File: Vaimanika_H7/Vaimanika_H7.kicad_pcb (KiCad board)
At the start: 4 copper layers, 40 x 40 mm, 64 parts, among them CN1 WAFER-GH1.25-3PWB, J1 TYPE-C 16PIN 2MD, J2 Conn_01x09, J3 Conn_01x09, J4 +VLIPO, J5 GND, J6 Conn_01x09, J8 Conn_01x02, Q1 AO3400A, Q2 AO3401A, U2 TPS54302, U3 USBLC6-2P6, U4 WAFER-GH1.25-4PWB, U5 WAFER-GH1.25-4PWB, U6 WAFER-GH1.25-4PWB, U7 WAFER-GH1.25-4PLB, U8 WAFER-GH1.25-4PLB, U9 WAFER-GH1.25-4PLB

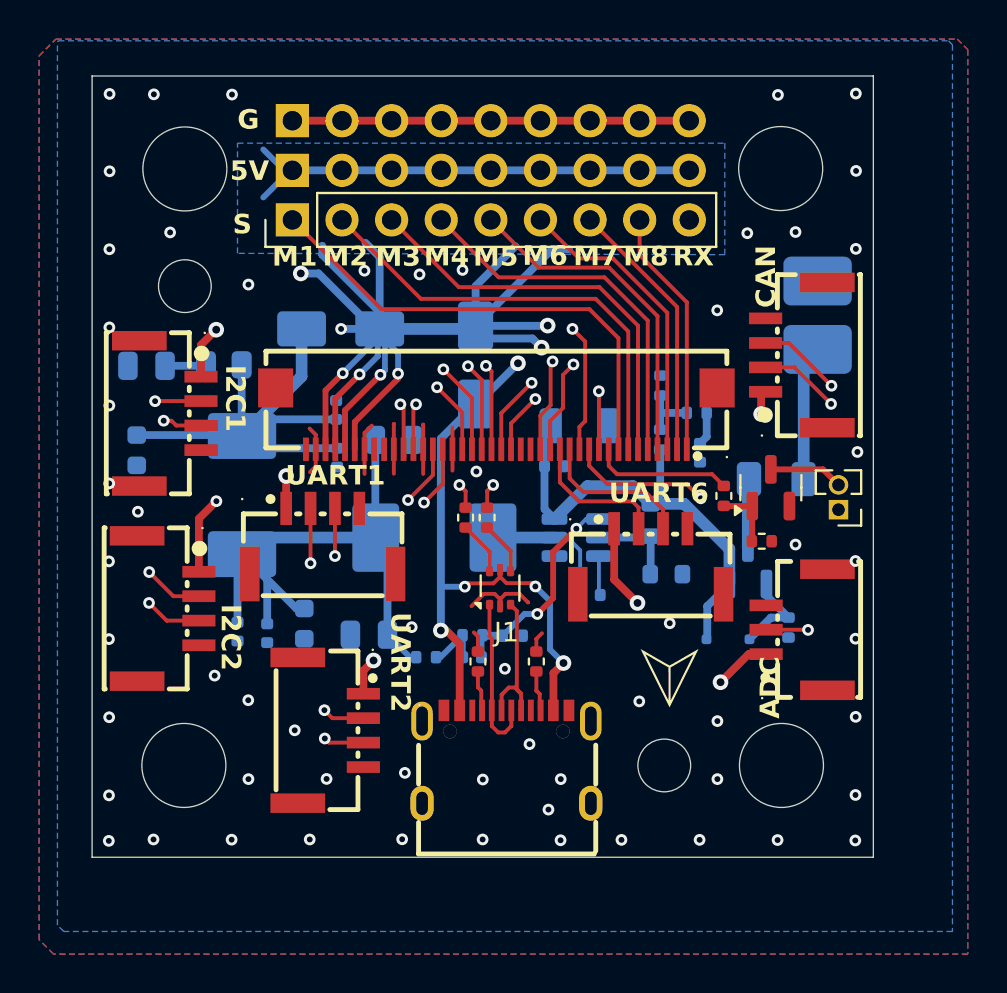
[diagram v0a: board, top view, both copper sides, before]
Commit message: Pilot PCB Done/03-06-2026
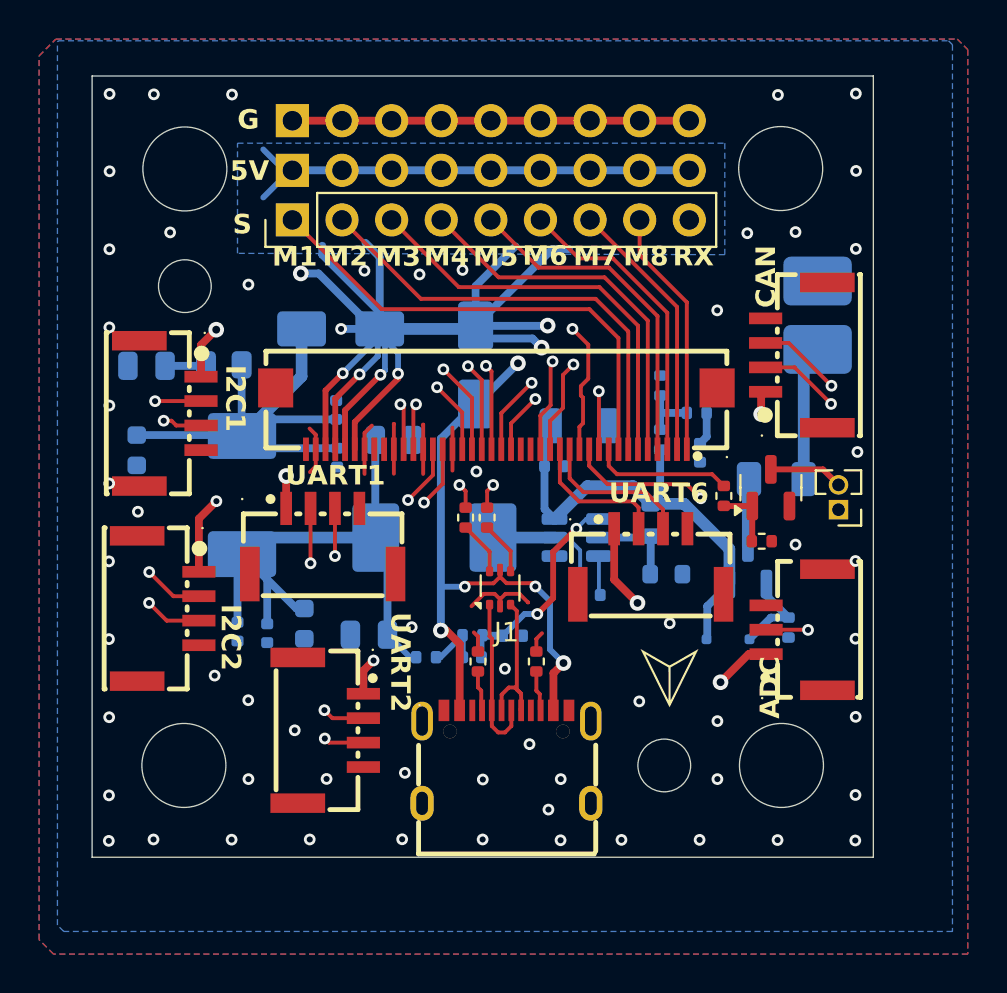
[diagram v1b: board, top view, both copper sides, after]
